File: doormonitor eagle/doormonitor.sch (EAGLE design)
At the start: 13 parts, among them Y1 8MHz

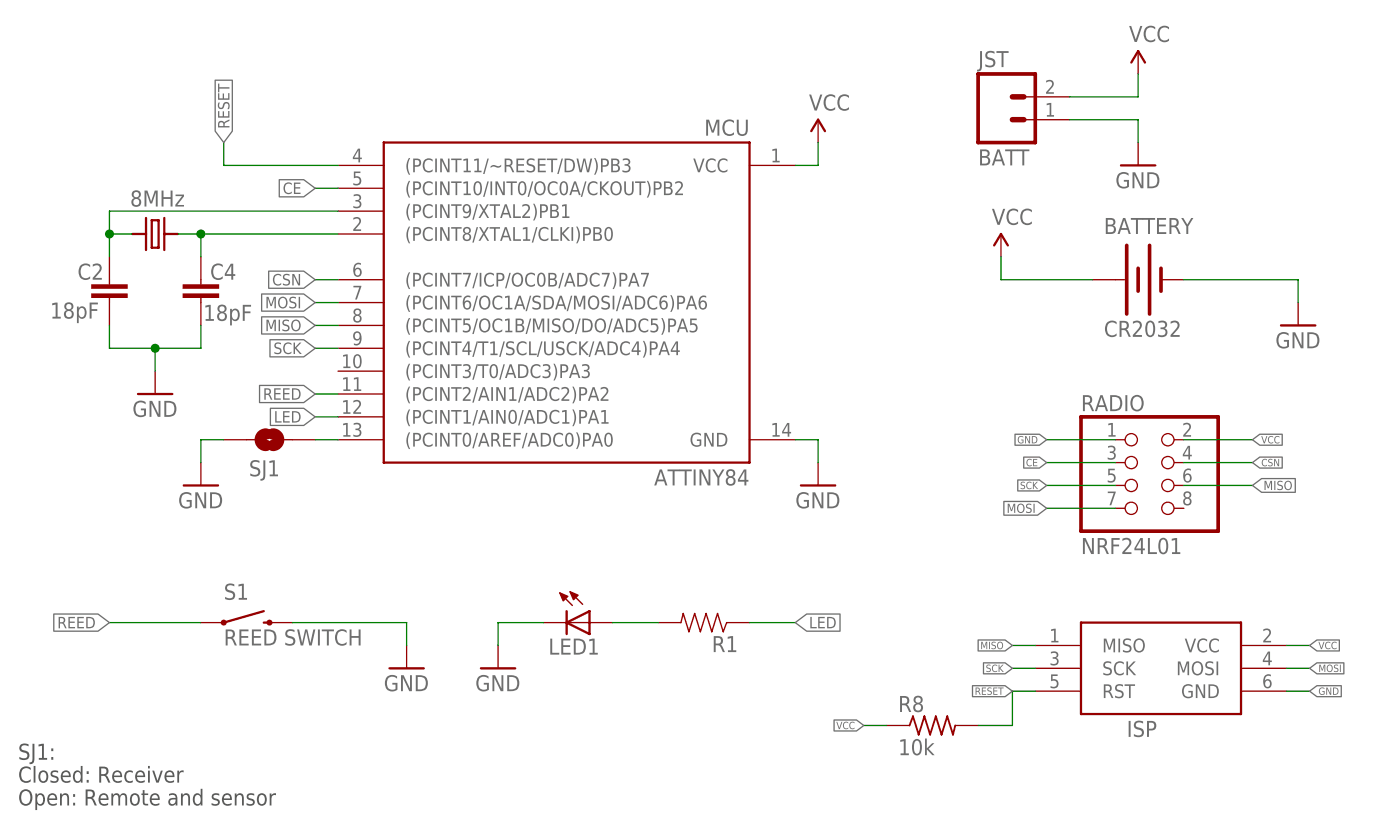
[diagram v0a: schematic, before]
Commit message: Fixing pinchange.
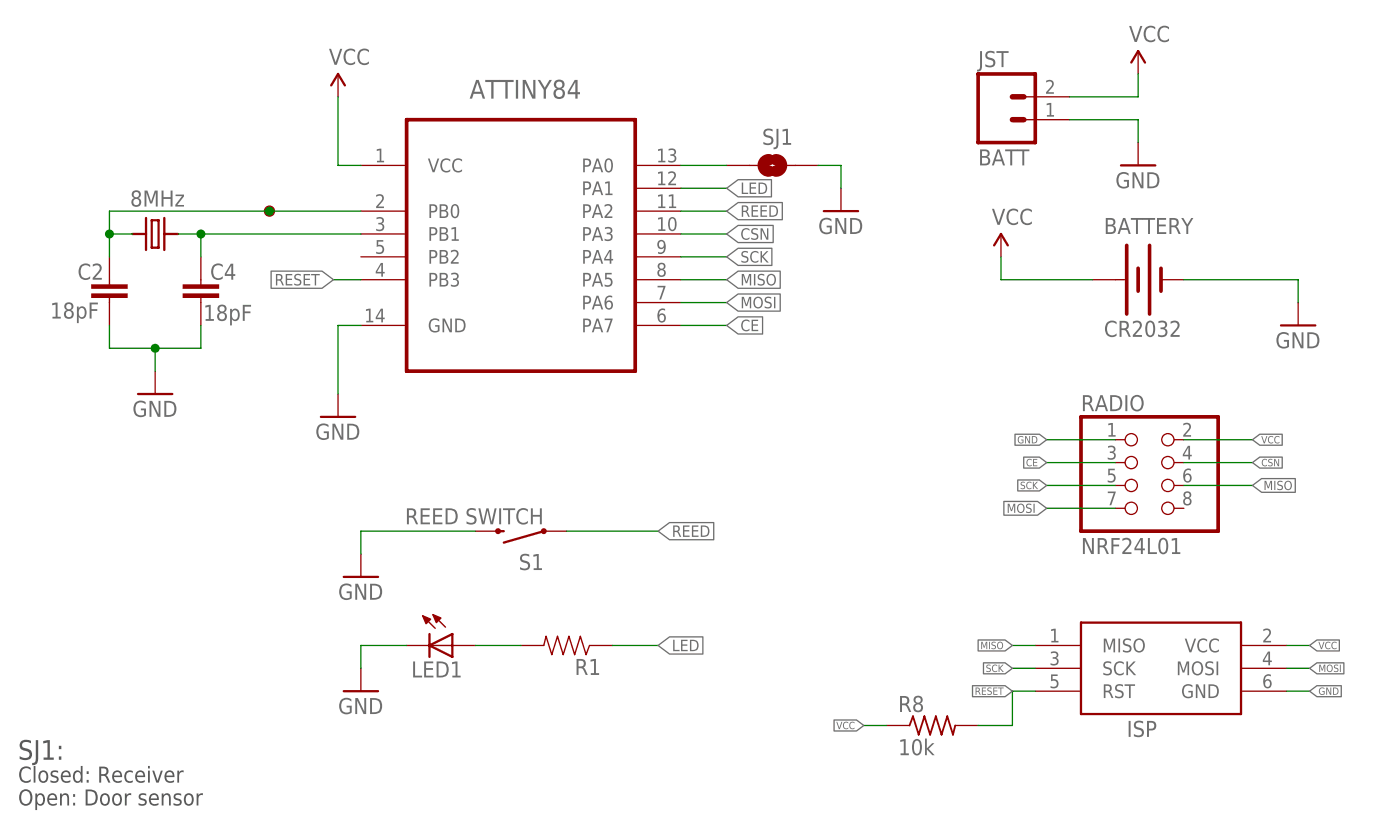
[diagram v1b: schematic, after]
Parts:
- removed MCU: ATTINY84, SparkFun-DigitalIC:ATTINY84
- added ATTINY84: ATTINY84-20SSU, Atmel_By_element14_Batch_1:ATTINY84-20SSU
- added U$1: VIA, thinkmaketest:VIA
- C2, C4: device SparkFun-Passives:CAP0402-CAP -> SparkFun-Passives:CAP0805
- LED1: device SparkFun-LED:LED10MM -> led:LED5MM
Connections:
- net CE: now also ATTINY84.PA7; no longer MCU.(PCINT10/INT0/OC0A/CKOUT)PB2
- net CSN: now also ATTINY84.PA3; no longer MCU.(PCINT7/ICP/OC0B/ADC7)PA7
- net GND: now also ATTINY84.GND; no longer MCU.GND
- net LED: now also ATTINY84.PA1; no longer MCU.(PCINT1/AIN0/ADC1)PA1
- net MISO: now also ATTINY84.PA5; no longer MCU.(PCINT5/OC1B/MISO/DO/ADC5)PA5
- net MOSI: now also ATTINY84.PA6; no longer MCU.(PCINT6/OC1A/SDA/MOSI/ADC6)PA6
- net N$2: now also ATTINY84.PA0; no longer MCU.(PCINT0/AREF/ADC0)PA0
- net N$3: now also ATTINY84.PB0, U$1.1; no longer MCU.(PCINT9/XTAL2)PB1
- net N$4: now also ATTINY84.PB1; no longer MCU.(PCINT8/XTAL1/CLKI)PB0
- net REED: now also ATTINY84.PA2; no longer MCU.(PCINT2/AIN1/ADC2)PA2
- net RESET: now also ATTINY84.PB3; no longer MCU.(PCINT11/~RESET/DW)PB3
- net SCK: now also ATTINY84.PA4; no longer MCU.(PCINT4/T1/SCL/USCK/ADC4)PA4
- net VCC: now also ATTINY84.VCC; no longer MCU.VCC
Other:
- note added: "Open: Door sensor"
- note removed: "Open: Remote and sensor"
- moved on the sheet: LED1, R1, S1, SJ1
